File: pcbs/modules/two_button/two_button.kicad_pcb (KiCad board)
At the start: 2 copper layers, 25.5 x 32 mm, 7 parts, among them SW1 SW_Push, SW2 SW_Push

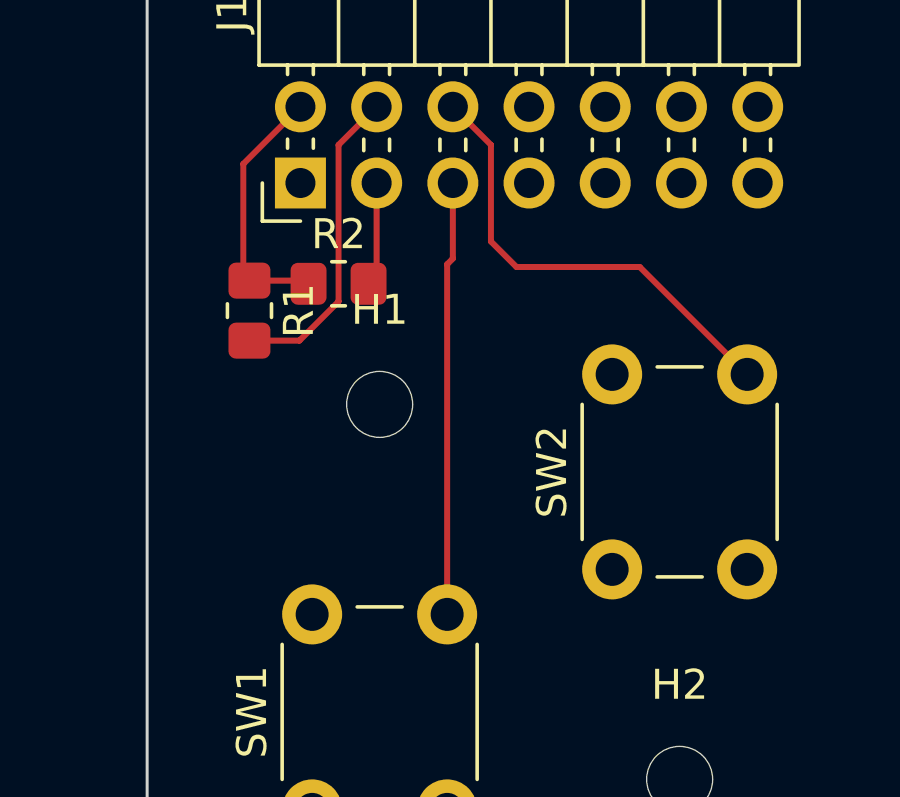
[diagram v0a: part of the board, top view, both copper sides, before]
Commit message: started to work on blender
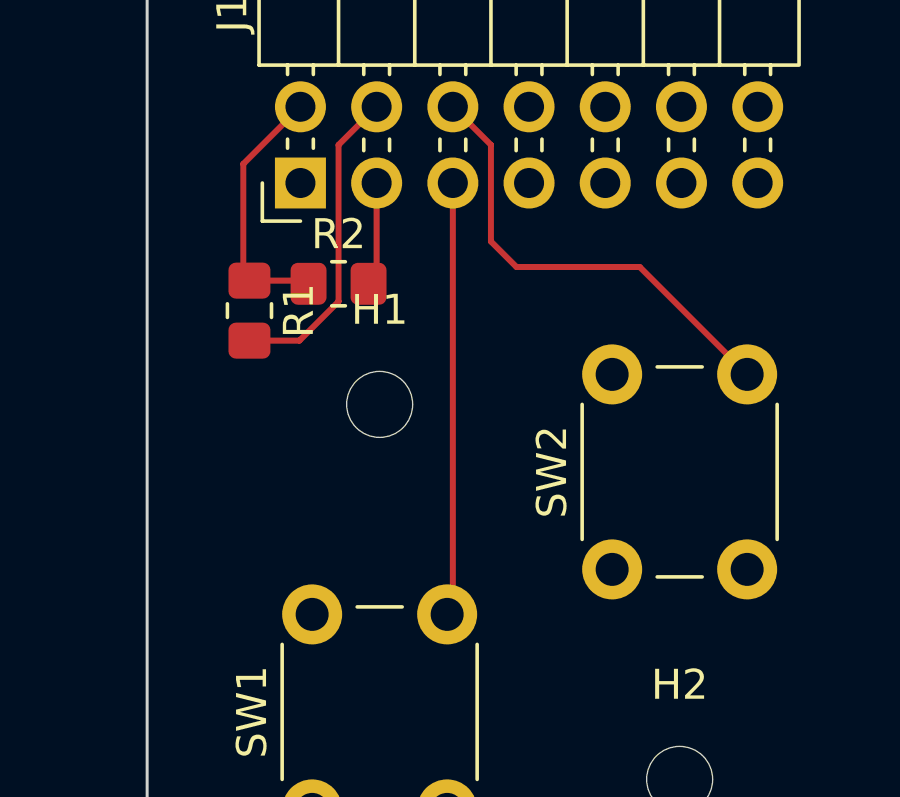
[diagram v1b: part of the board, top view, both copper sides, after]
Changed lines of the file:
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@@
 	)
 	(segment
-		(start 137.87 96.43)
-		(end 138.059999 96.240001)
-		(width 0.2)
-		(layer "F.Cu")
-		(net "/IO0")
-	)
-	(segment
-		(start 138.059999 96.240001)
+		(start 138.059999 107.91)
 		(end 138.059999 93.72)
 		(width 0.2)
@@
 	(segment
 		(start 137.87 108.099999)
-		(end 137.87 96.43)
+		(end 138.059999 107.91)
 		(width 0.2)
 		(layer "F.Cu")
